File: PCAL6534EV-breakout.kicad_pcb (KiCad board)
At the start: 6 copper layers, 15.2 x 50.8 mm, 21 parts, among them J1 SM04B-SRSS-TB, J2 Conn_01x20, J3 Conn_01x20, J4 Conn_02x04_Odd_Even, U1 PCAL6534EV

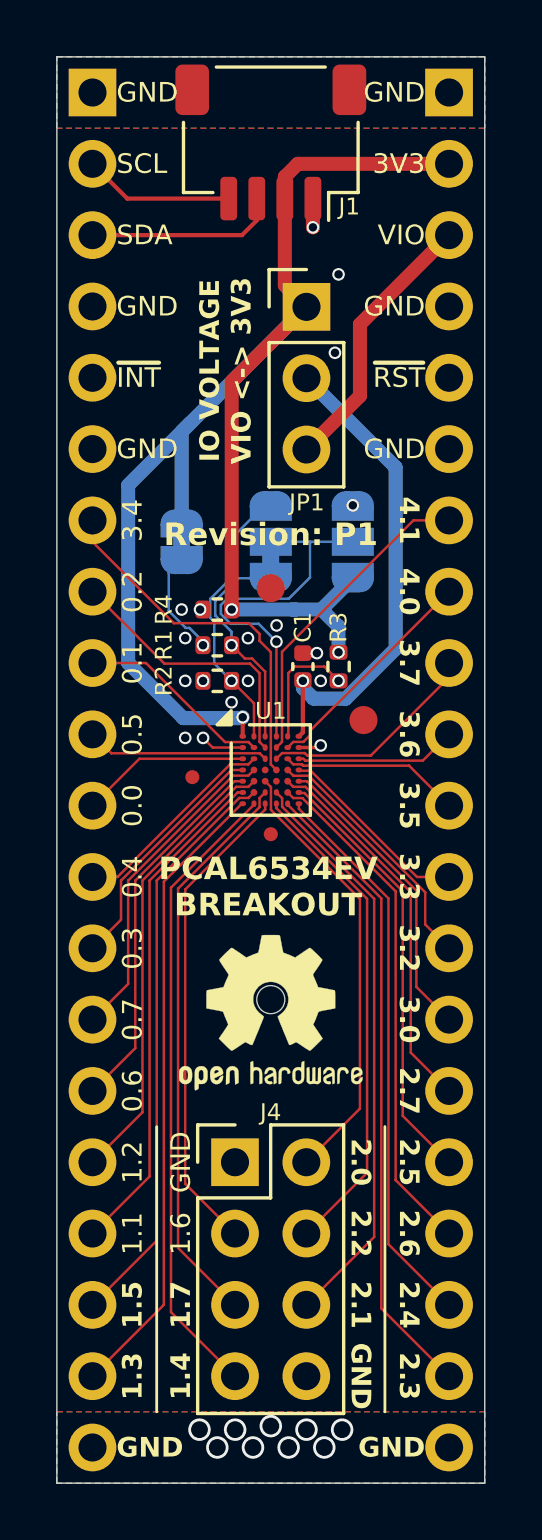
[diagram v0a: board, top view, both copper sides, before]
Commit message: nudge here, prod there, and pretty soon you've changed the entire thing
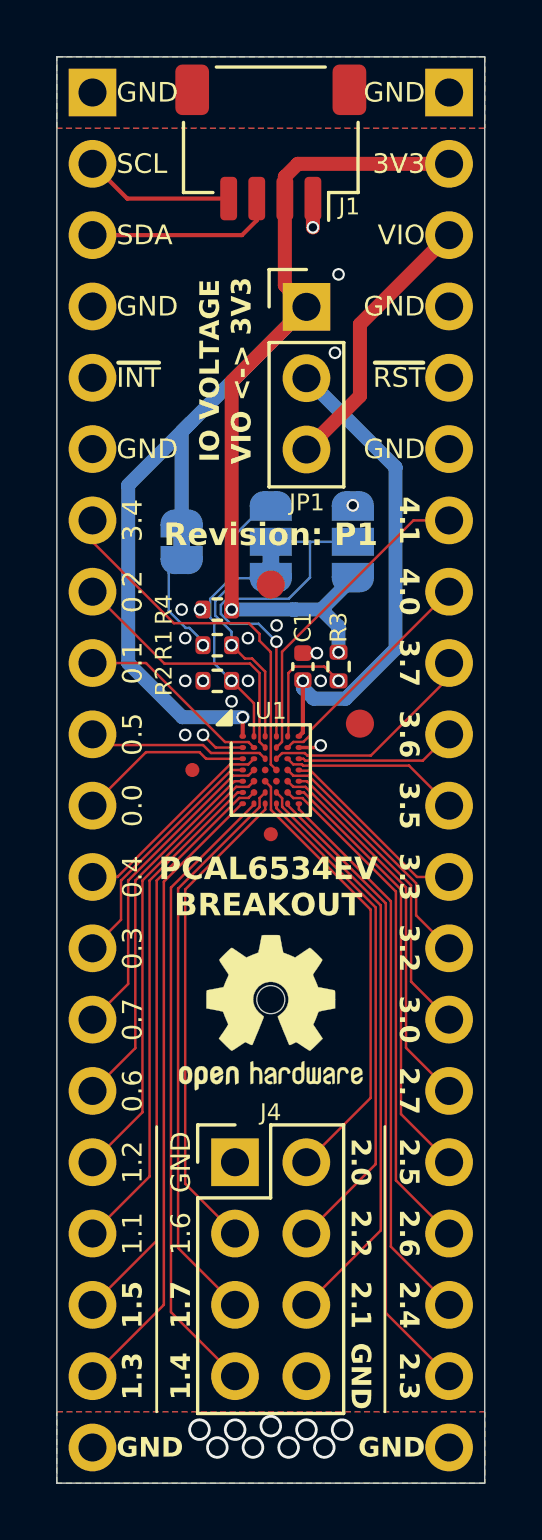
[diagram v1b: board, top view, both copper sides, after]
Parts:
- removed ? (x2): , 
- added FID3: Fiducial_1mm_Mask2mm, Fiducial:Fiducial_1mm_Mask2mm, F.Cu at (155.0, 103.9)
- added FID4: Fiducial_1mm_Mask2mm, Fiducial:Fiducial_1mm_Mask2mm, F.Cu at (158.2, 108.8)
- moved FID1 0.25 mm to (152.2, 110.5)
- renumbered REF** to FID1, REF** to FID2

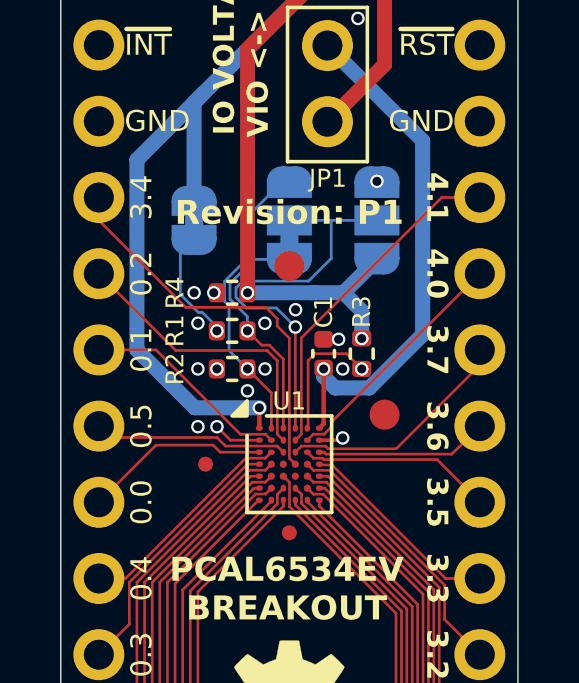
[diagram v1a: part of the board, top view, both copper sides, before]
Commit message: just slam them all in an update again
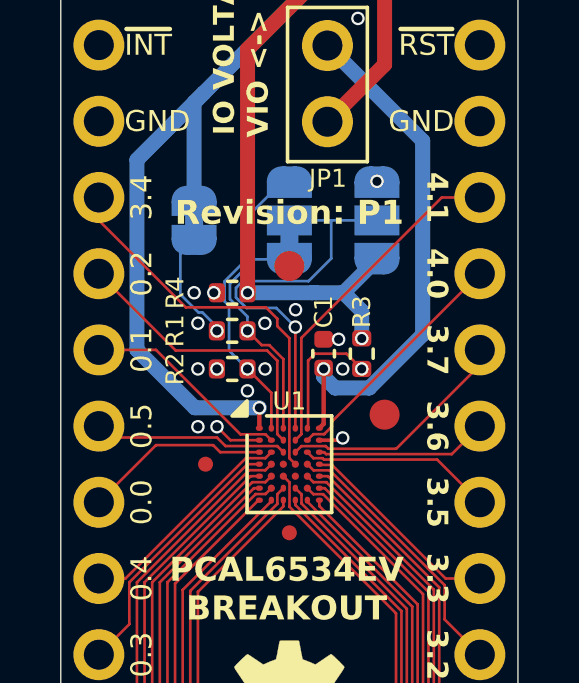
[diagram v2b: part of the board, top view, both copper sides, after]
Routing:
- net P3_4: track 13.2 -> 12.4 mm
- net P0_5: track 6.51 -> 5.97 mm
- net P3_7: track 7.93 -> 7.42 mm
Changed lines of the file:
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@@
-	)
-	(segment
-		(start 149.031 109.591)
-		(end 148.65 109.21)
-		(width 0.09)
-		(layer "F.Cu")
-		(net 5)
 	)
 	(segment
@@
 	)
 	(segment
-		(start 154.4 111.68)
-		(end 154.4 111.715)
-		(width 0.09)
-		(layer "F.Cu")
-		(net 9)
-	)
-	(segment
 		(start 154.4 111.715)
 		(end 151.444 114.671)
@@
 	)
 	(segment
-		(start 148.65 102.353117)
-		(end 148.65 101.59)
-		(width 0.09)
-		(layer "F.Cu")
-		(net 10)
-	)
-	(segment
 		(start 155 110.28)
 		(end 155 106.27894)
@@
 	)
 	(segment
-		(start 155.6 111.68)
-		(end 155.6 111.731214)
-		(width 0.09)
-		(layer "F.Cu")
-		(net 11)
-	)
-	(segment
 		(start 159.096 115.227214)
 		(end 159.095997 129.815997)
@@
 	)
 	(segment
-		(start 161.35 107.178)
-		(end 161.35 106.67)
-		(width 0.09)
-		(layer "F.Cu")
-		(net 17)
-	)
-	(segment
 		(start 156.025 110.505)
 		(end 156.422 110.505)
@@
 	)
 	(segment
-		(start 156 110.48)
-		(end 156.025 110.505)
-		(width 0.09)
-		(layer "F.Cu")
-		(net 18)
-	)
-	(segment
 		(start 155.6 109.68)
 		(end 155.8 109.48)
@@
 		(layer "F.Cu")
 		(net 28)
-	)
-	(segment
-		(start 154 111.68)
-		(end 153.97 111.68)
-		(width 0.09)
-		(layer "F.Cu")
-		(net 29)
 	)
 	(segment
@@
 	)
 	(segment
-		(start 153.607 104.762988)
-		(end 153.607 104.765)
-		(width 0.5)
-		(layer "B.Cu")
-		(net 34)
-	)
-	(segment
 		(start 157.413 106.289)
 		(end 157.413 105.37)
@@
 	)
 	(segment
-		(start 154.78 101.052)
-		(end 155 101.052)
-		(width 0.09)
-		(layer "B.Cu")
-		(net 35)
-	)
-	(segment
 		(start 153.603 107.305)
 		(end 152.989002 106.691002)
@@
 	)
 	(segment
-		(start 156.01 109.27)
-		(end 156 109.27)
-		(width 0.15)
-		(layer "F.Cu")
-		(net 37)
-	)
-	(segment
 		(start 156.143 109.137)
 		(end 156.01 109.27)
@@
 	)
 	(segment
-		(start 157.394 107.235)
-		(end 157.413 107.305)
-		(width 0.09)
-		(layer "F.Cu")
-		(net 41)
-	)
-	(segment
 		(start 156.905 106.797)
 		(end 155.855106 106.797)
@@
 		(width 0.09)
 		(layer "F.Cu")
-		(net 41)
-	)
-	(segment
-		(start 155.624998 109.255002)
-		(end 155.6 109.28)
-		(width 0.09)
-		(layer "F.Cu")
